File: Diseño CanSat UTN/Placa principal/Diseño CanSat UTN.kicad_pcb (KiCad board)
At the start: 2 copper layers, 60 x 60 mm, 11 parts, among them J1 Jack-DC, J2 Conn_01x15_MountingPin, J3 Conn_01x15_MountingPin, U1 L7805, U2 MicroSD-Card-Adapter

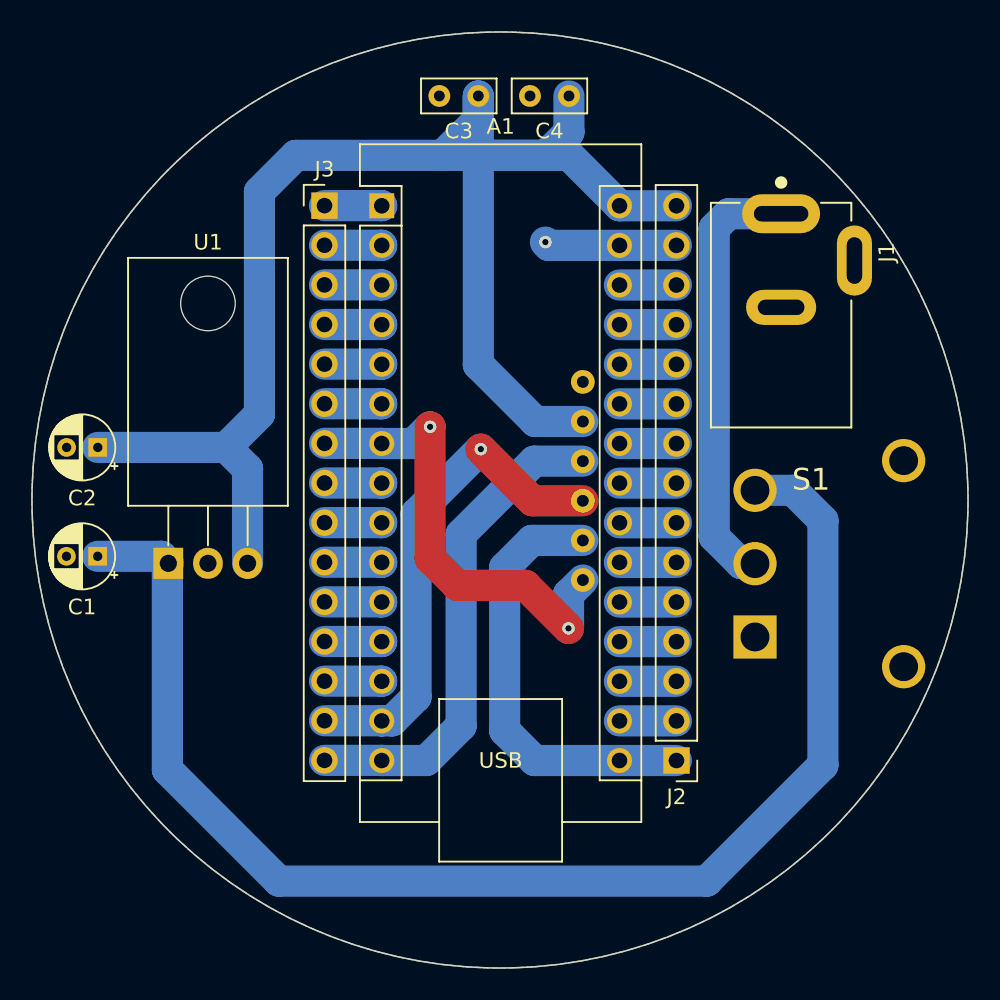
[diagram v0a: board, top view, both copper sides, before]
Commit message: ACTUALIZACION
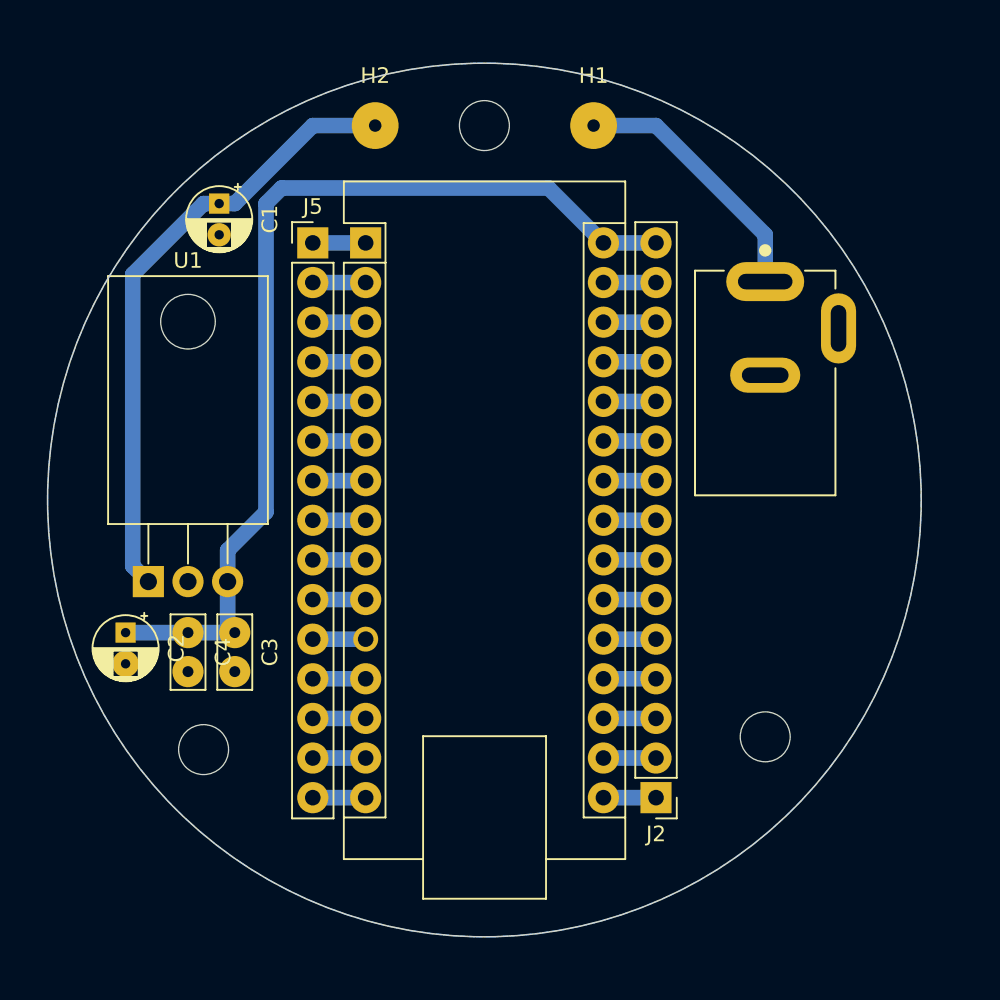
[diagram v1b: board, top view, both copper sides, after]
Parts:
- removed J3: Conn_01x15_MountingPin, Connector_PinHeader_2.54mm:PinHeader_1x15_P2.54mm_Vertical
- removed S1: Switch-Horizontal, Switch-Horizontal:Switch-Horizontal-2
- removed U2: MicroSD-Card-Adapter, MicroSD-Card-Adapter:MicroSD-Card-Adapter
- added H1: MountingHole_Pad, MountingHole:MountingHole_2.2mm_M2_Pad, F.Cu at (156.0, 76.0)
- added H2: MountingHole_Pad, MountingHole:MountingHole_2.2mm_M2_Pad, F.Cu at (142.0, 76.0)
- added J5: Conn_01x15_MountingPin, Connector_PinHeader_2.54mm:PinHeader_1x15_P2.54mm_Vertical, F.Cu at (138.0, 83.5)
- added REF**: MountingHole_3.2mm_M3, MountingHole:MountingHole_3.2mm_M3, F.Cu at (131.0, 116.0)
- added REF**: MountingHole_3.2mm_M3, MountingHole:MountingHole_3.2mm_M3, F.Cu at (149.0, 76.0)
- added REF**: MountingHole_3.2mm_M3, MountingHole:MountingHole_3.2mm_M3, F.Cu at (167.0, 115.2)
- moved C4 42.2 mm to (130.0, 108.5), turned to -90 degrees
- moved C3 37.8 mm to (133.0, 108.5), turned to -90 degrees
- moved C1 23.9 mm to (132.0, 81.0), turned to -90 degrees
- moved C2 12.0 mm to (126.0, 108.5), turned to -90 degrees
- moved J1 4.47 mm to (167.0, 86.0)
- moved J2 2.72 mm to (160.0, 119.1)
- moved A1 2.59 mm to (141.4, 83.5)
- moved U1 1.73 mm to (127.5, 105.2)
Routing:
- net Net-(U1-IN): track 86.8 -> 39.6 mm
- net +5V: track 106.8 -> 62.6 mm
- net /Arduino Nano/14: track 32.0 -> 3.39 mm, vias 1 -> 0
- net /Arduino Nano/15: track 31.7 -> 3.39 mm
- net /Arduino Nano/7: track 29.9 -> 3.39 mm, vias 2 -> 0
- net /Arduino Nano/16: track 28.0 -> 3.37 mm
- net +9V: track 27.8 -> 16.9 mm
- net GND: track 12.2 -> 6.76 mm, vias 1 -> 0
- removed copper zone on F.Cu, net GND
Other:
- board size 60 x 60 mm -> 56 x 56 mm
